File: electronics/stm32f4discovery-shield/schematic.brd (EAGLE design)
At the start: 100 x 80 mm, 1 part

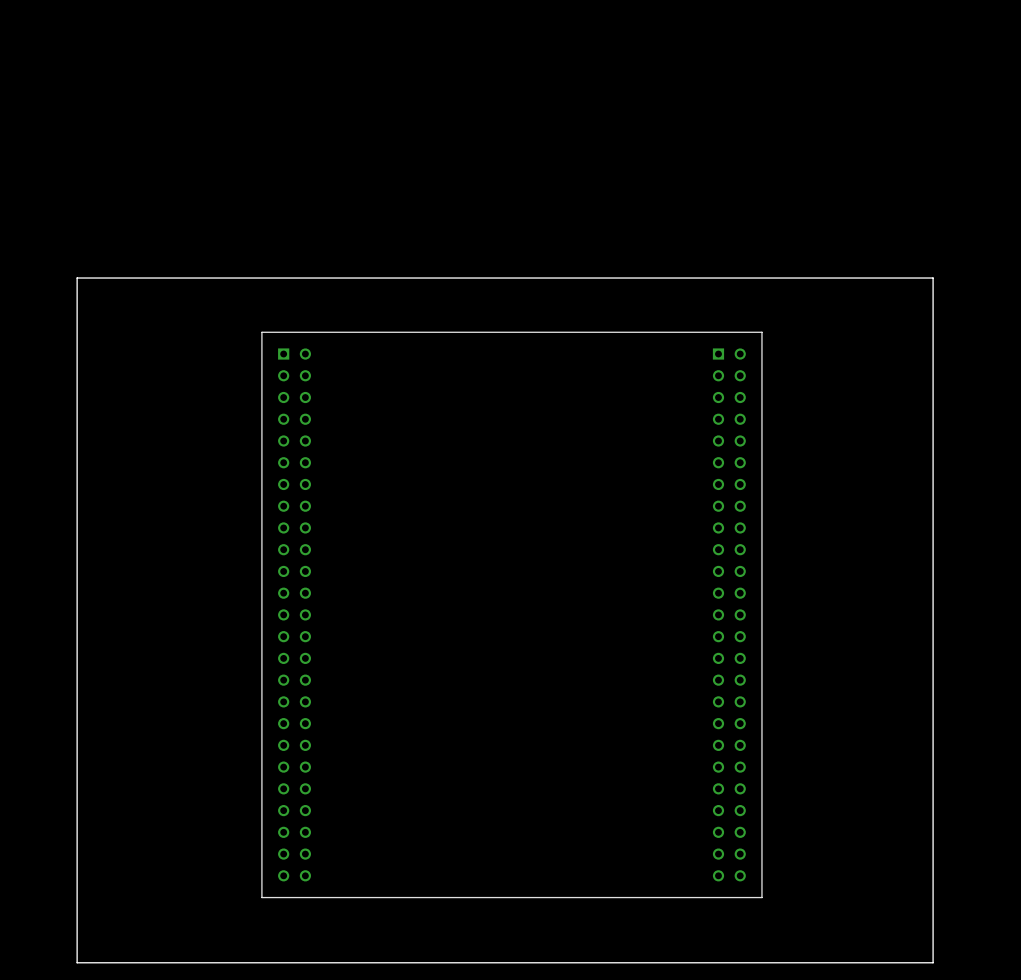
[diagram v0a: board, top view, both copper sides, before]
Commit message: Iniciando o routing.
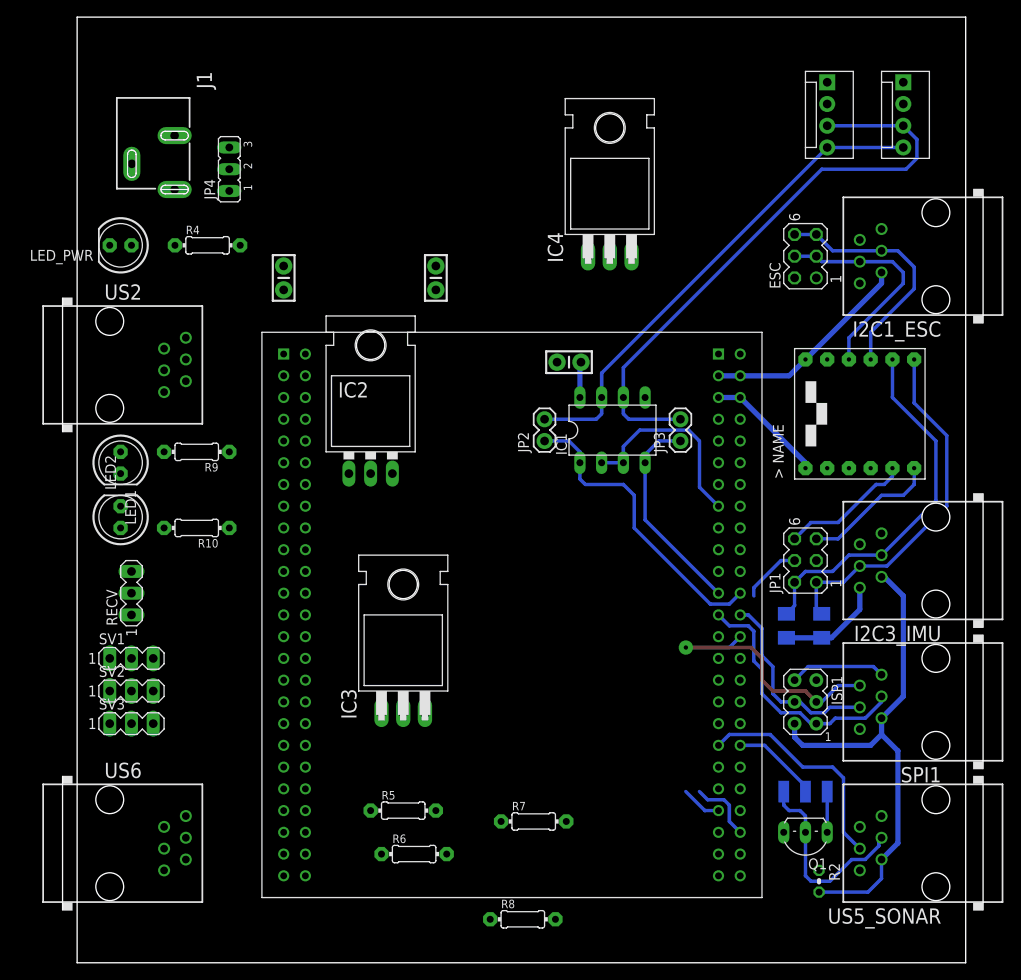
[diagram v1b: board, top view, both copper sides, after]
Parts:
- added C1: 104, SparkFun-Capacitors:CAP-PTH-SMALL-KIT
- added C2, C3: (no value), SparkFun-Capacitors:CAP-PTH-SMALL-KIT
- added ESC, JP1: (no value), con-lstb:MA03-2
- added I2C1_ESC, I2C3_IMU, SPI1, US2, US5_SONAR, US6: RJ11-2L-B, con-tycoelectronics:RJ11-NO_SHIELD
- added IC1: MAX3468CPA, maxim:DIL08
- added IC2: (no value), SparkFun-PowerIC:TO-220-ALT
- added IC3, IC4: LM340H-12, linear:TO220H
- added ISP1: AVRISP-6, adafruit:AVRISP
- added J1: POWER_JACKSLT, SparkFun-Connectors:POWER_JACK_SLOT
- added JP2, JP3: (no value), SparkFun-Passives:1X02
- added JP4: (no value), jumper:JP2
- added LED1, LED2, LED_PWR: (no value), adafruit:LED5MM
- added Q1: BC548, transistor-npn:TO92-EBC
- added R1, R3: (no value), adafruit:M1206
- added R10, R4, R5, R6, R7, R8, R9: (no value), adafruit:0204/7
- added R2: (no value), rcl:0204V
- added RECV, SV1, SV2, SV3: (no value), con-lstb:MA03-1
- added SJ1: (no value), jumper:SJ_2W
- added SRVO1, SRVO2: (no value), SparkFun-Connectors:MOLEX-1X4
- added U$2: JYMCU_LOGIC_LEVEL_CONVERTER, provant_custom:JYMCU_LOGIC_LEVEL_SHIFTER_DIP
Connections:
- new net 3.3V: I2C1_ESC.1, I2C3_IMU.1, R1.2, R3.2, U$1.P$55, U$1.P$56, U$2.3V3, US2.1, US5_SONAR.1, US6.1
- new net 5V: C1.1, I2C1_ESC.2, I2C3_IMU.2, IC1.8, ISP1.2, JP4.2, R10.1, R2.2, R4.2, R9.1, RECV.2, SPI1.2, SV1.2, SV2.2, SV3.2, U$1.P$53, U$1.P$54, U$2.5V, US2.2, US5_SONAR.2, US6.2
- new net 5V_REG: C3.1, IC2.OUT, JP4.1
- new net D+/TX: IC1.6, JP3.2, SRVO1.3, SRVO2.3
- new net D-/RX: IC1.7, JP2.2, SRVO1.4, SRVO2.4
- new net GND: C1.2, C2.2, C3.2, ESC.1, ESC.2, I2C1_ESC.5, I2C1_ESC.6, I2C3_IMU.5, I2C3_IMU.6, IC1.5, IC2.GND, ISP1.6, J1.GND@1, J1.GND@2, LED_PWR.K, Q1.E, R6.2, R8.2, RECV.3, SPI1.6, SRVO1.1, SRVO2.1, SV1.3, SV2.3, SV3.3, U$1.P$1, U$1.P$100, U$1.P$2, U$1.P$23, U$1.P$49, U$1.P$5, U$1.P$50, U$1.P$51, U$1.P$52, U$1.P$99, U$2.GND1, U$2.GND2, US2.5, US2.6, US5_SONAR.5, US5_SONAR.6, US6.5, US6.6
- new net N$1: JP1.5, U$2.DL
- new net N$2: JP1.6, U$2.CL
- new net N$3: Q1.C, R2.1, SJ1.3
- new net N$4: LED_PWR.A, R4.1
- new net N$5: LED1.A, R9.2
- new net N$6: IC3.2, R5.1, R6.1
- new net N$7: LED2.A, R10.2
- new net N$8: IC4.2, R7.2, R8.1
- new net PA2/USART2_TX: U$1.P$14, US2.3
- new net PA3/USART2_RX: U$1.P$13, US2.4
- new net PA8/I2C3_SCL: JP1.4, U$1.P$93
- new net PB0/PWM: LED2.K
- new net PB1/PWM: LED1.K
- new net PB3/SPI1_SCK: ISP1.3, SPI1.5, U$1.P$78
- new net PB4/SPI1_MISO: ISP1.1, SPI1.4, U$1.P$75
- new net PB5/SPI1_MOSI: ISP1.4, SPI1.3, U$1.P$76
- new net PB6/USART1_TX: IC1.4, JP3.1, U$1.P$73
- new net PB7/USART1_RX: IC1.1, JP2.1, U$1.P$74
- new net PB8/I2C1_SCL: U$1.P$69, U$2.BL
- new net PB9/I2C1_SDA: U$1.P$70, U$2.AL
- new net PC10/USART3_TX: U$1.P$87, US5_SONAR.3
- new net PC11/USART3_RX: SJ1.2, U$1.P$88
- new net PC6/USART6_TX: U$1.P$97, US6.3
- new net PC7/USART6_RX: U$1.P$98, US6.4
- new net PC9/I2C3_SDA: JP1.3, U$1.P$96
- new net PE11/PWM: SV3.1
- new net PE13/PWM: SV2.1
- new net PE14/PWM: SV1.1
- new net PE2: IC1.2, IC1.3, U$1.P$65
- new net PE9/PWM: RECV.1
- new net SCL1: ESC.5, ESC.6, I2C1_ESC.4, U$2.BH
- new net SCL2: I2C3_IMU.4, JP1.2, R3.1, U$2.CH
- new net SDA1: ESC.3, ESC.4, I2C1_ESC.3, U$2.AH
- new net SDA2: I2C3_IMU.3, JP1.1, R1.1, U$2.DH
- new net SONAR_RX: Q1.B, SJ1.1, US5_SONAR.4
- new net SRVO1_PWR: IC4.3, R7.1, SRVO1.2
- new net SRVO2_PWR: IC3.3, R5.2, SRVO2.2
- new net VCC: C2.1, IC2.IN, IC3.1, IC4.1, J1.PWR, JP4.3
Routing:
- net 5V: track 0.00 -> 88.7 mm
- net D+/TX: track 0.00 -> 70.1 mm
- net D-/RX: track 0.00 -> 57.9 mm
- net SCL2: track 0.00 -> 43.1 mm
- net SDA2: track 0.00 -> 41.6 mm
- net PB7/USART1_RX: track 0.00 -> 35.4 mm
- net PB3/SPI1_SCK: track 0.00 -> 31.5 mm, vias 0 -> 1
- net PB4/SPI1_MISO: track 0.00 -> 29.7 mm
- net SCL1: track 0.00 -> 28.4 mm
- net 3.3V: track 0.00 -> 26.4 mm
- net SDA1: track 0.00 -> 26.3 mm
- net PC10/USART3_TX: track 0.00 -> 26.3 mm
- net PB6/USART1_TX: track 0.00 -> 24.5 mm
- net SONAR_RX: track 0.00 -> 23.3 mm
- net PE2: track 0.00 -> 23.2 mm
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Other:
- board size 100 x 80 mm -> 103.8 x 110.5 mm
